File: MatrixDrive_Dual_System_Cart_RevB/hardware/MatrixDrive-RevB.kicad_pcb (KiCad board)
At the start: 2 copper layers, 100 x 65 mm, 25 parts, among them J1 MEGA_DRIVE_EDGE_VERIFY_ORIENT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, J2 USB-C, J4 CPLD JTAG, SW1 PROGRAM, SW2 MD / SMS, SW3 SMS PAUSE, SW4 SEGA / CODEMASTERS, U1 RP2350B QFN80, U10 STAGING SPI, U11 3V3 LDO, U13 ATF1508ASV CPLD, U14 CTRL2 XCVR, U15-U16 DATA CONTROL, U17 32KiB FRAM LOW, U18 32KiB FRAM HIGH, U2 S29GL032N TSOP48, U3 ADDR XCVR 0-7, U4 ADDR XCVR 8-15, U5 ADDR/CTRL XCVR, U6 LOW DATA BIDI, U7 HIGH DATA OUT, U9 BOOT QSPI, Y1 12MHz

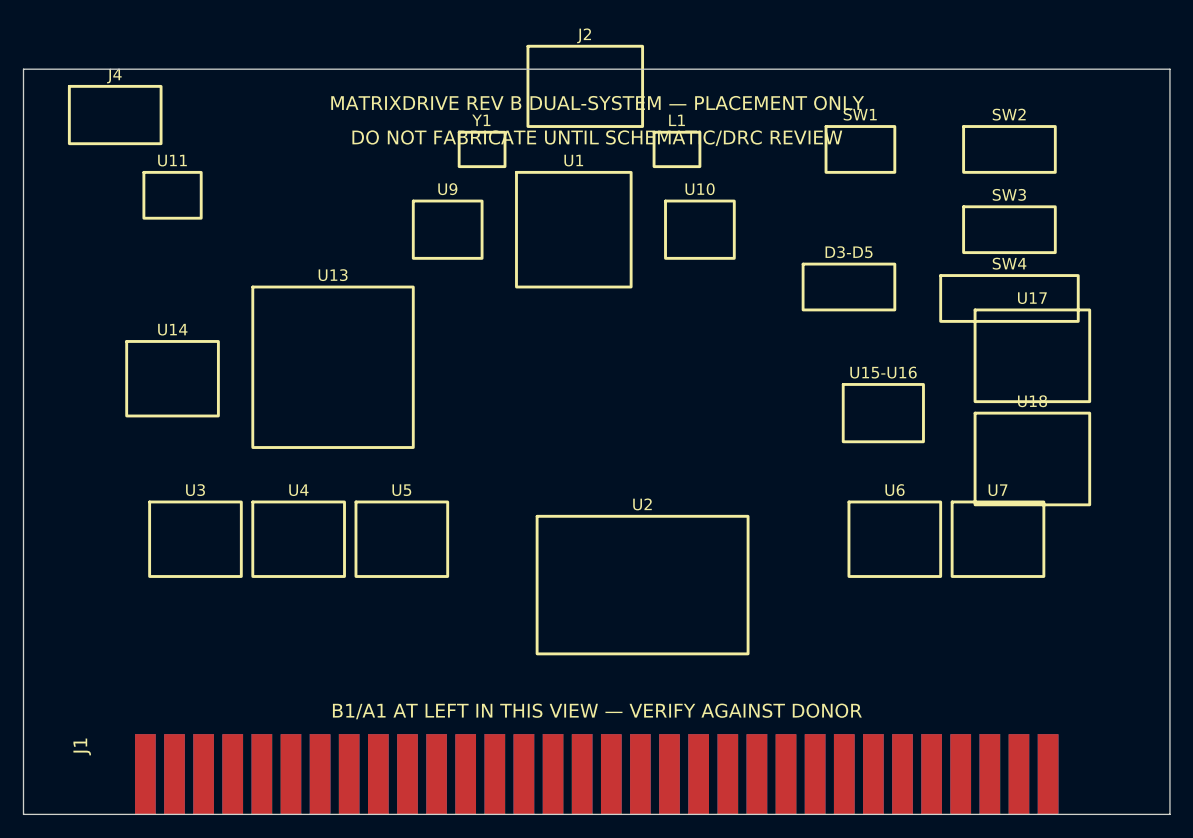
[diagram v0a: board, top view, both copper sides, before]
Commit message: Regenerate lock-on PCB template and package [skip ci]
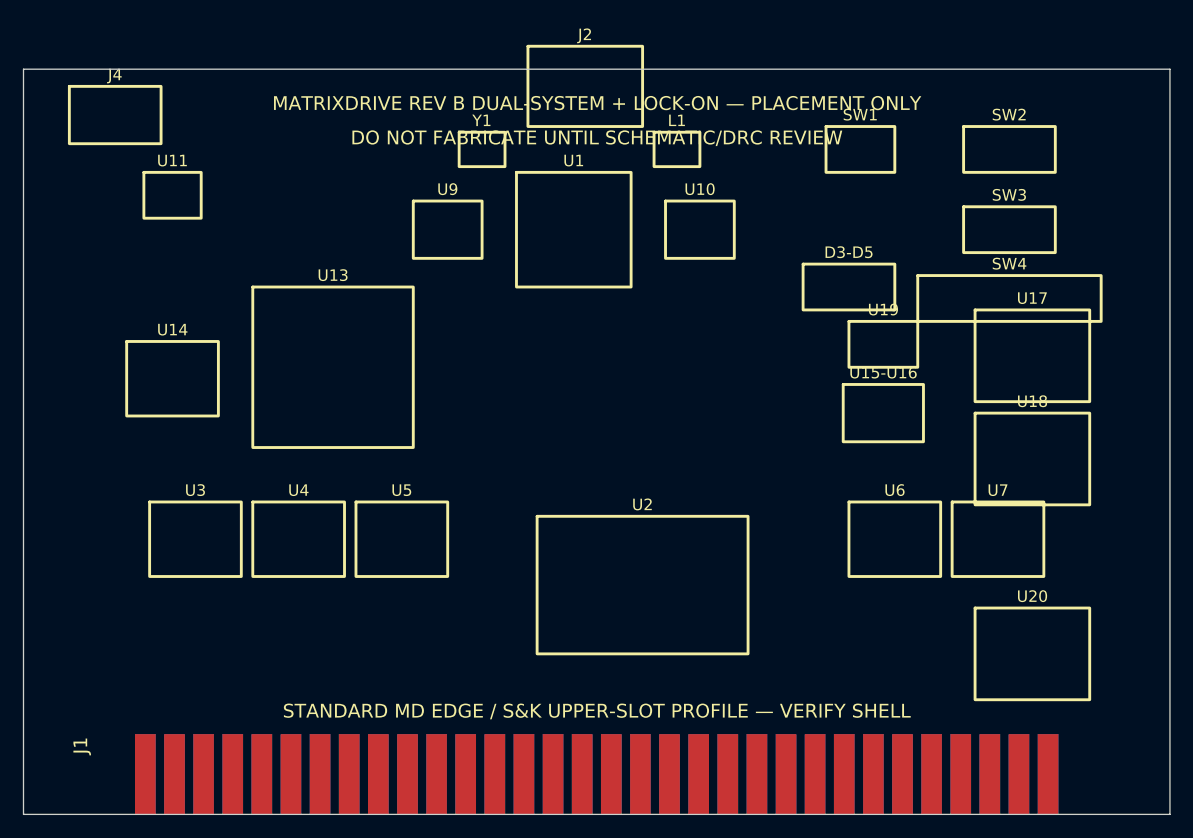
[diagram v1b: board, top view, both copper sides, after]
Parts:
- added U19: MD HIGH DISABLE XCVR, MatrixDrive:PLACEMENT_U19, F.Cu at (75.0, 24.0)
- added U20: SONIC 3 SAVE FRAM, MatrixDrive:PLACEMENT_U20, F.Cu at (88.0, 51.0)
- SW4: value SEGA / CODEMASTERS -> SEGA-LINEAR / CODIES-S3 SAVE
- U15-U16: value DATA CONTROL -> DATA CONTROL ORS
- U17: value 32KiB FRAM LOW -> 32KiB SMS FRAM LOW
- U18: value 32KiB FRAM HIGH -> 32KiB SMS FRAM HIGH
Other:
- board text added: "MATRIXDRIVE REV B DUAL-SYSTEM + LOCK-ON — PLACEMENT ONLY"
- board text added: "STANDARD MD EDGE / S&K UPPER-SLOT PROFILE — VERIFY SHELL"
- board text removed: "B1/A1 AT LEFT IN THIS VIEW — VERIFY AGAINST DONOR"
- board text removed: "MATRIXDRIVE REV B DUAL-SYSTEM — PLACEMENT ONLY"
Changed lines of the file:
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@@
   (setup (pad_to_mask_clearance 0))
   (gr_rect (start 0 0) (end 100 65) (stroke (width 0.10) (type default)) (fill none) (layer "Edge.Cuts"))
-  (gr_text "MATRIXDRIVE REV B DUAL-SYSTEM — PLACEMENT ONLY" (at 50.00 3.00) (layer "F.SilkS")
+  (gr_text "MATRIXDRIVE REV B DUAL-SYSTEM + LOCK-ON — PLACEMENT ONLY" (at 50.00 3.00) (layer "F.SilkS")
     (effects (font (size 1.20 1.20) (thickness 0.20)))
   )
@@
     (fp_text reference "U15-U16" (at 0 -3.50) (layer "F.SilkS")
       (effects (font (size 1 1) (thickness 0.15))))
-    (fp_text value "DATA CONTROL" (at 0 0) (layer "F.Fab")
+    (fp_text value "DATA CONTROL ORS" (at 0 0) (layer "F.Fab")
       (effects (font (size 0.8 0.8) (thickness 0.12))))
   )
@@
     (fp_text reference "U17" (at 0 -5.00) (layer "F.SilkS")
       (effects (font (size 1 1) (thickness 0.15))))
-    (fp_text value "32KiB FRAM LOW" (at 0 0) (layer "F.Fab")
+    (fp_text value "32KiB SMS FRAM LOW" (at 0 0) (layer "F.Fab")
       (effects (font (size 0.8 0.8) (thickness 0.12))))
   )
@@
     (fp_text reference "U18" (at 0 -5.00) (layer "F.SilkS")
       (effects (font (size 1 1) (thickness 0.15))))
-    (fp_text value "32KiB FRAM HIGH" (at 0 0) (layer "F.Fab")
+    (fp_text value "32KiB SMS FRAM HIGH" (at 0 0) (layer "F.Fab")
+      (effects (font (size 0.8 0.8) (thickness 0.12))))
+  )
+  (footprint "MatrixDrive:PLACEMENT_U19" (layer "F.Cu") (at 75.00 24.00)
+    (attr board_only exclude_from_pos_files exclude_from_bom)
+    (fp_rect (start -3.00 -2.00) (end 3.00 2.00)
+      (stroke (width 0.25) (type default)) (fill none) (layer "F.SilkS"))
+    (fp_text reference "U19" (at 0 -3.00) (layer "F.SilkS")
+      (effects (font (size 1 1) (thickness 0.15))))
+    (fp_text value "MD HIGH DISABLE XCVR" (at 0 0) (layer "F.Fab")
+      (effects (font (size 0.8 0.8) (thickness 0.12))))
+  )
+  (footprint "MatrixDrive:PLACEMENT_U20" (layer "F.Cu") (at 88.00 51.00)
+    (attr board_only exclude_from_pos_files exclude_from_bom)
+    (fp_rect (start -5.00 -4.00) (end 5.00 4.00)
+      (stroke (width 0.25) (type default)) (fill none) (layer "F.SilkS"))
+    (fp_text reference "U20" (at 0 -5.00) (layer "F.SilkS")
+      (effects (font (size 1 1) (thickness 0.15))))
+    (fp_text value "SONIC 3 SAVE FRAM" (at 0 0) (layer "F.Fab")
       (effects (font (size 0.8 0.8) (thickness 0.12))))
   )
@@
   (footprint "MatrixDrive:PLACEMENT_SW4" (layer "F.Cu") (at 86.00 20.00)
     (attr board_only exclude_from_pos_files exclude_from_bom)
-    (fp_rect (start -6.00 -2.00) (end 6.00 2.00)
+    (fp_rect (start -8.00 -2.00) (end 8.00 2.00)
       (stroke (width 0.25) (type default)) (fill none) (layer "F.SilkS"))
     (fp_text reference "SW4" (at 0 -3.00) (layer "F.SilkS")
       (effects (font (size 1 1) (thickness 0.15))))
-    (fp_text value "SEGA / CODEMASTERS" (at 0 0) (layer "F.Fab")
+    (fp_text value "SEGA-LINEAR / CODIES-S3 SAVE" (at 0 0) (layer "F.Fab")
       (effects (font (size 0.8 0.8) (thickness 0.12))))
   )
@@
       (effects (font (size 0.8 0.8) (thickness 0.12))))
   )
-  (gr_text "B1/A1 AT LEFT IN THIS VIEW — VERIFY AGAINST DONOR" (at 50.00 56.00) (layer "F.SilkS")
+  (gr_text "STANDARD MD EDGE / S&K UPPER-SLOT PROFILE — VERIFY SHELL" (at 50.00 56.00) (layer "F.SilkS")
     (effects (font (size 1.20 1.20) (thickness 0.20)))
   )
